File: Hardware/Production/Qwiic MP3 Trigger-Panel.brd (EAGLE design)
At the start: 115.6 x 115.8 mm, 636 parts, among them J1 MICRO-SD, J13 PTH, J14 QWIIC_RIGHT_ANGLE, J2 QWIIC_RIGHT_ANGLE, J20 MICRO-SD, J21 ISP, J22 Poke-Home, J23 3.5mm Audio, J25 QWIIC_RIGHT_ANGLE, J26 PTH, J27 QWIIC_RIGHT_ANGLE, J3 PTH, J32 MICRO-SD, J33 ISP, J34 Poke-Home, J35 3.5mm Audio, J37 QWIIC_RIGHT_ANGLE, J38 PTH, J39 QWIIC_RIGHT_ANGLE, J4 QWIIC_RIGHT_ANGLE, J44 MICRO-SD, J45 ISP, J46 Poke-Home, J47 3.5mm Audio, J49 QWIIC_RIGHT_ANGLE, J50 PTH, J51 QWIIC_RIGHT_ANGLE, J56 MICRO-SD, J57 ISP, J58 Poke-Home, J59 3.5mm Audio, J6 QWIIC_RIGHT_ANGLE, J61 QWIIC_RIGHT_ANGLE, J62 PTH, J63 QWIIC_RIGHT_ANGLE, J68 MICRO-SD, J69 ISP, J7 ISP, J70 Poke-Home, J71 3.5mm Audio, J8 3.5mm Audio, J9 Poke-Home, U1 TPA2005D1, U10 ATTINY84-ARDUINO, U11 AP2112-3.3V, U12 WT2003SH4, U13 TPA2005D1, U14 ATTINY84-ARDUINO, U15 AP2112-3.3V, U16 WT2003SH4, U17 TPA2005D1, U18 ATTINY84-ARDUINO, U19 AP2112-3.3V, U2 TPA2005D1, U20 WT2003SH4, U21 TPA2005D1, U22 ATTINY84-ARDUINO, U23 AP2112-3.3V, U24 WT2003SH4, U3 AP2112-3.3V, U4 ATTINY84-ARDUINO, U5 WT2003SH4, U6 ATTINY84-ARDUINO, U7 AP2112-3.3V, U8 WT2003SH4, U9 TPA2005D1

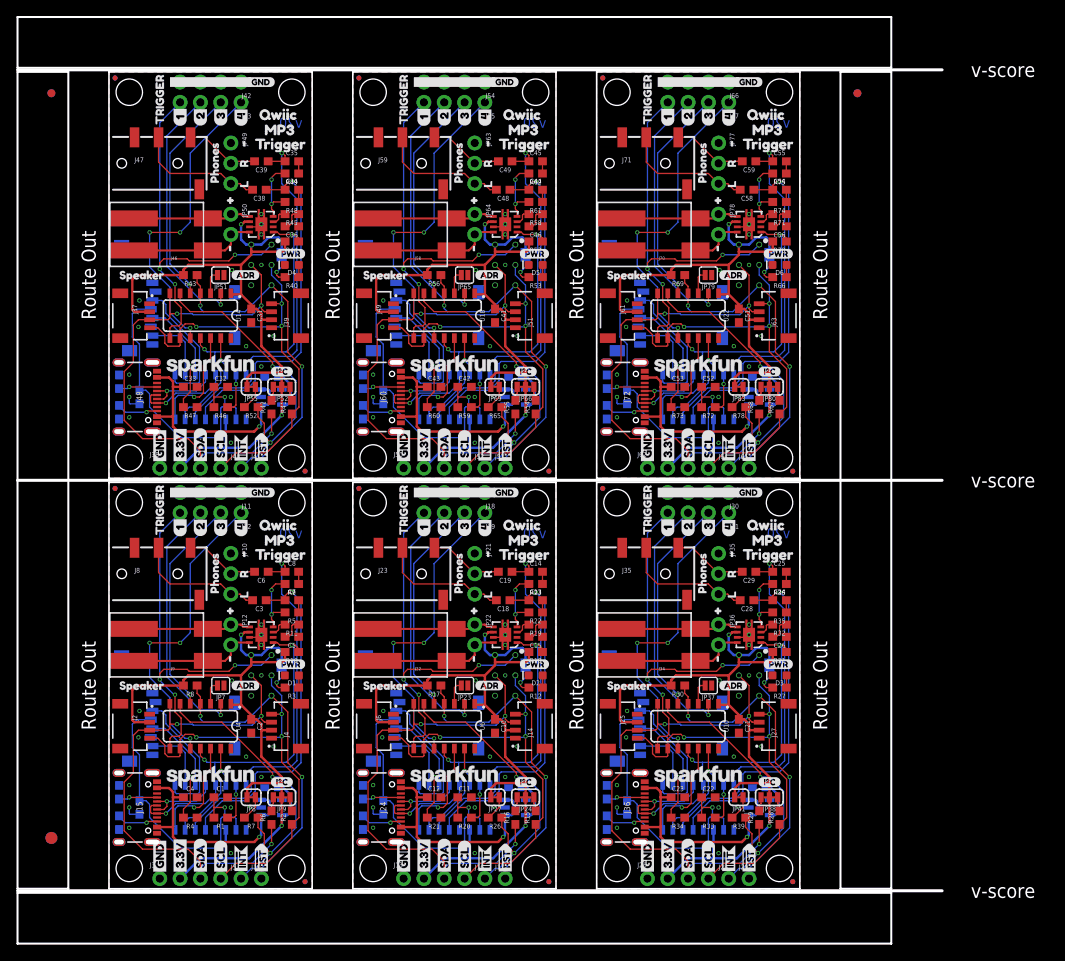
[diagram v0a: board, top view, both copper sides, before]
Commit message: v20 small test panel
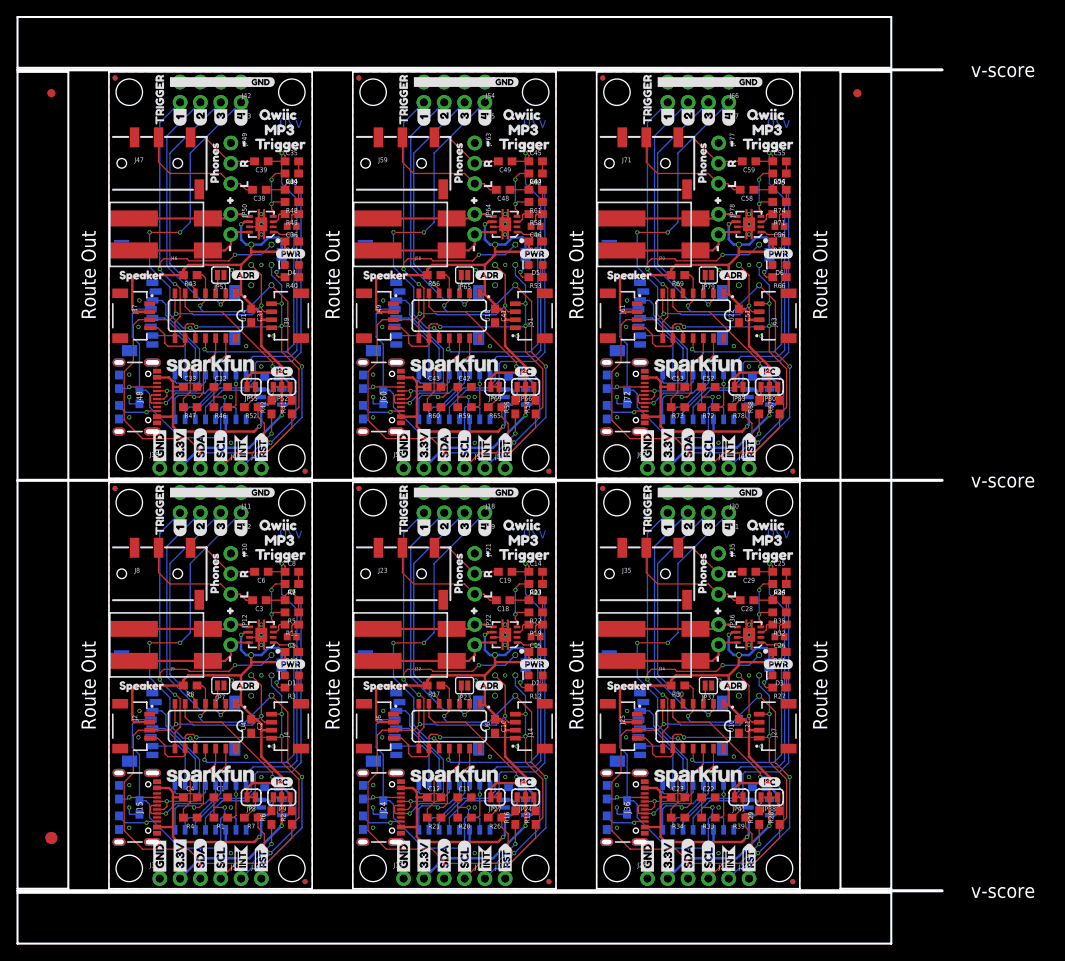
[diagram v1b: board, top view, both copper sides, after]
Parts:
- C13, C14, C24, C25, C34, C35, C44, C45, C54, C55, C7, C8: value 0.1uF -> 10nF
- C15, C26, C36, C46, C5, C56: value 1.0uF -> 22nF; device SparkFun-Capacitors:0603 -> SparkFun-Capacitors:0402
- R11, R19, R32, R45, R58, R71: value 100k -> 47k
- R17, R30, R43, R56, R69, R8: value 4.7k -> 10k
- R22, R23, R35, R36, R48, R49, R5, R61, R62, R74, R75, R9: value 10k -> 100k
- moved U10 0.64 mm to (73.0, 20.3)
- moved U18 0.64 mm to (42.5, 71.6)
- moved U22 0.64 mm to (73.0, 71.6)
- moved U6 0.64 mm to (42.5, 20.3)
- moved U14 0.63 mm to (12.1, 71.6)
- moved U4 0.63 mm to (12.1, 20.3)
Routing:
- net !RST2: track 41.3 -> 42.2 mm
- net !RST1: track 41.3 -> 42.2 mm
- net !RST5: track 41.3 -> 42.2 mm
- net !RST4: track 41.3 -> 42.2 mm
- net !RST3: track 41.3 -> 42.2 mm
- net !RST: track 41.3 -> 42.2 mm
- net TRIGGER22: track 48.7 -> 47.9 mm
- net TRIGGER10: track 48.7 -> 47.9 mm
- net TRIGGER1: track 48.7 -> 47.9 mm
- net TRIGGER6: track 48.7 -> 47.9 mm
- net TRIGGER18: track 48.7 -> 47.9 mm
- net TRIGGER14: track 48.7 -> 47.9 mm
- net 3.3V3: track 94.9 -> 94.2 mm
- net 3.3V2: track 94.9 -> 94.2 mm
- net 3.3V: track 94.9 -> 94.2 mm
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
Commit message: Proto with MY1690
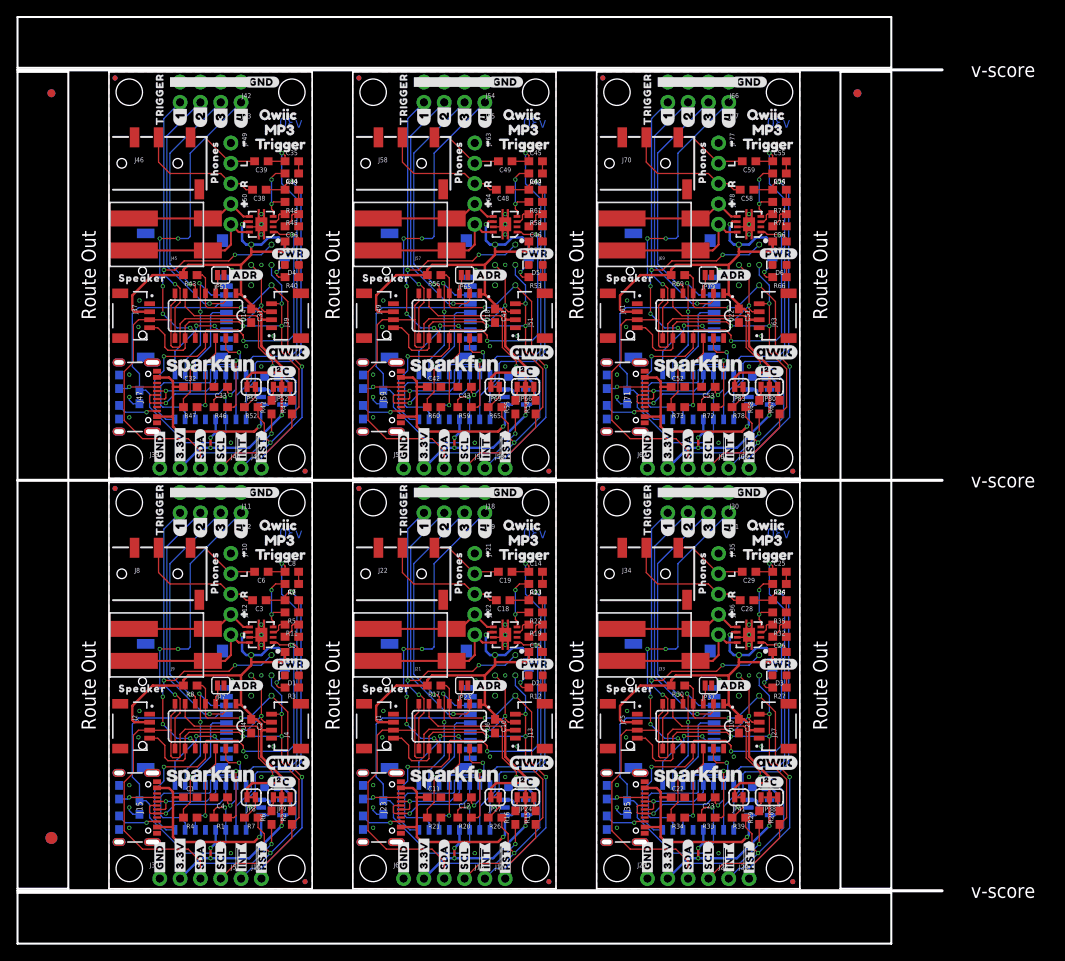
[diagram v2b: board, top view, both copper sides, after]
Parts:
- removed U$283: (no value), Labels:QWIIC-LOGO-MEDIUM
- removed U$284: (no value), buzzard_labels (2):TRIGGER4
- removed U$285: (no value), buzzard_labels (3):MP31
- removed U$286: (no value), buzzard_labels (3):QWIIC0
- removed U$287: (no value), buzzard_labels (3):TRIGGER2
- removed U$288: (no value), output:#PWR#0
- added LOGO19, LOGO23: SFE_LOGO_NAME_FLAME.1_INCH, SparkFun-Aesthetics:SFE_LOGO_NAME_FLAME_.1
- added LOGO20, LOGO24: QWIIC_LOGO_CONNECTOR, SparkFun-Aesthetics:QWIIC_5.5MM
- added LOGO21: OSHW-LOGOMINI, SparkFun-Aesthetics:OSHW-LOGO-MINI
- added LOGO22: SFE_LOGO_NAME.1_INCH, SparkFun-Aesthetics:SFE_LOGO_NAME_.1
- C1, C11, C22, C32, C42, C52: value 10uF -> 1.0uF
- C15, C26, C36, C46, C5, C56: device SparkFun-Capacitors:0402 -> SparkFun-Capacitors:0603
- J1: value MICRO-SD -> QWIIC_RIGHT_ANGLE; device SparkFun-Connectors:MICRO-SD-SOCKET -> SparkFun-Connectors:JST04_1MM_RA
- J13: value PTH -> QWIIC_RIGHT_ANGLE; device SparkX:1X04_NO_SILK -> SparkFun-Connectors:JST04_1MM_RA
- J14: value QWIIC_RIGHT_ANGLE -> MICRO-SD; device SparkFun-Connectors:JST04_1MM_RA -> SparkFun-Connectors:MICROSD-EXTERNALPIN
- J20, J32, J44, J56, J68: value MICRO-SD -> ISP; device SparkFun-Connectors:MICRO-SD-SOCKET -> SparkFun-Connectors:2X3_TEST_POINTS
- J21, J33, J45, J57, J69: value ISP -> Poke-Home; device SparkFun-Connectors:2X3_TEST_POINTS -> SparkFun-Connectors:1X02_POKEHOME
- J22, J34, J46, J58, J70: value Poke-Home -> 3.5mm Audio; device SparkFun-Connectors:1X02_POKEHOME -> SparkFun-Connectors:AUDIO_JACK_3.5MM_TRRS_SMD_RA
- J23, J35, J47, J59, J71: value 3.5mm Audio -> (none); device SparkFun-Connectors:AUDIO_JACK_3.5MM_TRRS_SMD_RA -> SparkFun-Connectors:USB-C-16P-2LAYER-PADS
- J24, J36, J48, J60, J72: value (none) -> MICRO-SD; device SparkFun-Connectors:USB-C-16P-2LAYER-PADS -> SparkFun-Connectors:MICROSD-EXTERNALPIN
- J6: value QWIIC_RIGHT_ANGLE -> PTH; device SparkFun-Connectors:JST04_1MM_RA -> SparkX:1X04_NO_SILK
- LOGO10: value OSHW-LOGOMINI -> SFE_LOGO_NAME.1_INCH; device SparkFun-Aesthetics:OSHW-LOGO-MINI -> SparkFun-Aesthetics:SFE_LOGO_NAME_.1
- LOGO11: value SFE_LOGO_NAME.1_INCH -> SFE_LOGO_NAME_FLAME.1_INCH; device SparkFun-Aesthetics:SFE_LOGO_NAME_.1 -> SparkFun-Aesthetics:SFE_LOGO_NAME_FLAME_.1
- LOGO12: value SFE_LOGO_NAME_FLAME.1_INCH -> QWIIC_LOGO_CONNECTOR; device SparkFun-Aesthetics:SFE_LOGO_NAME_FLAME_.1 -> SparkFun-Aesthetics:QWIIC_5.5MM
- LOGO16, LOGO4: value OSHW-LOGOMINI -> QWIIC_LOGO_CONNECTOR; device SparkFun-Aesthetics:OSHW-LOGO-MINI -> SparkFun-Aesthetics:QWIIC_5.5MM
- LOGO17, LOGO5: value SFE_LOGO_NAME.1_INCH -> OSHW-LOGOMINI; device SparkFun-Aesthetics:SFE_LOGO_NAME_.1 -> SparkFun-Aesthetics:OSHW-LOGO-MINI
- LOGO18, LOGO6: value SFE_LOGO_NAME_FLAME.1_INCH -> SFE_LOGO_NAME.1_INCH; device SparkFun-Aesthetics:SFE_LOGO_NAME_FLAME_.1 -> SparkFun-Aesthetics:SFE_LOGO_NAME_.1
- LOGO7: value OSHW-LOGOMINI -> SFE_LOGO_NAME_FLAME.1_INCH; device SparkFun-Aesthetics:OSHW-LOGO-MINI -> SparkFun-Aesthetics:SFE_LOGO_NAME_FLAME_.1
- LOGO8: value SFE_LOGO_NAME.1_INCH -> QWIIC_LOGO_CONNECTOR; device SparkFun-Aesthetics:SFE_LOGO_NAME_.1 -> SparkFun-Aesthetics:QWIIC_5.5MM
- LOGO9: value SFE_LOGO_NAME_FLAME.1_INCH -> OSHW-LOGOMINI; device SparkFun-Aesthetics:SFE_LOGO_NAME_FLAME_.1 -> SparkFun-Aesthetics:OSHW-LOGO-MINI
- U$10, U$38, U$69: device buzzard_labels (16):#6 -> output:#1#3
- U$100, U$148: device Labels-0_04:SDA8 -> output:#0
- U$101, U$194, U$242: device Labels-0_04:GND1 -> output:#0
- U$102, U$150: device Labels-0_04:3#3V2 -> output:#1
- U$103, U$196, U$244: device Labels-0_04:SDA8 -> output:#1
- U$104: device Labels-0_04:SCL9 -> output:QWIIC_MP30
- U$105: device Labels:I_SUPER2_C-()-03 -> output:TRIGGER1
- U$106: device Labels:INT#-[< -> output:#PWR#0
- U$107, U$154, U$155, U$202: device Labels:INT#-[< -> output:TRIGGER0
- U$108: device Labels:RST#-[> -> output:TRIGGER0
- U$109, U$156, U$157, U$204: device Labels:RST#-[> -> output:L1
- U$11: device Labels:INT#-[< -> output:#1
- U$110: device Labels:PWR-()-03 -> output:L1
- U$111, U$159: device Labels:ADR-()-03 -> output:R0
- U$112, U$64: device buzzard_labels (13):TRIGGER5 -> output:R0
- U$113, U$161: device buzzard_labels (14):21 -> output:#2
- U$114, U$66: device buzzard_labels (14):32 -> output:#2
- U$115, U$163: device buzzard_labels (14):43 -> output:#1#3
- U$116, U$68: device buzzard_labels (16):#5 -> output:#1#3
- U$117, U$165: device buzzard_labels (16):#6 -> output:#2#2
- U$118, U$70: device buzzard_labels (16):1_1 -> output:#2#2
- U$119, U$167: device buzzard_labels (16):GND0 -> output:#3#1
- U$12, U$28: device buzzard_labels (16):#5 -> output:#1
- U$120, U$72: device buzzard_labels (16):L12 -> output:#3#1
- U$121, U$169: device buzzard_labels (16):R11 -> output:#4#0
- U$122, U$74: device buzzard_labels (16):#6 -> output:#4#0
- U$123, U$171: device buzzard_labels (17):PHONES0 -> output:#GND#0
- U$124, U$76: device buzzard_labels (17):SPEAKER1 -> output:#GND#0
- U$125: device buzzard_labels (17):QWIIC_MP32 -> output:PHONES0
- U$126: device buzzard_labels (16):#6 -> output:#PWR#0
- U$127: device buzzard_labels (16):#5 -> output:#ADR#0
- U$128: device buzzard_labels (14):43 -> output:SPEAKER0
- U$129: device buzzard_labels (14):32 -> output:#I�C#0
- U$13: device buzzard_labels (16):#6 -> output:#1
- U$130, U$178: device buzzard_labels (16):#6 -> output:##INT##4
- U$131, U$83: device buzzard_labels (16):R11 -> output:##INT##4
- U$132, U$180: device buzzard_labels (16):L12 -> output:##RST##5
- U$133, U$85: device buzzard_labels (14):21 -> output:##RST##5
- U$134, U$182, U$44: device buzzard_labels (16):1_1 -> output:#3#3V#0
- U$135, U$87: device buzzard_labels (13):TRIGGER5 -> output:#3#3V#0
- U$136, U$184, U$46: device buzzard_labels (16):GND0 -> output:#GND#1
- U$137, U$89: device buzzard_labels (17):PHONES0 -> output:#GND#1
- U$138, U$186: device buzzard_labels (17):SPEAKER1 -> output:#SCL#3
- U$139, U$91: device Labels:QWIIC-LOGO-MEDIUM -> output:#SCL#3
- U$14: device buzzard_labels (17):SPEAKER1 -> output:#0
- U$140, U$188: device buzzard_labels (2):TRIGGER4 -> output:#SDA#2
- U$141, U$93: device buzzard_labels (3):MP31 -> output:#SDA#2
- U$142: device buzzard_labels (3):QWIIC0 -> buzzard_labels (3):MP31
- U$143: device buzzard_labels (3):TRIGGER2 -> buzzard_labels (3):QWIIC0
- U$144: device output:#PWR#0 -> buzzard_labels (3):TRIGGER2
- U$145: device Labels-0_04:3#3V2 -> output:PHONES0
- U$146: device Labels-0_04:GND1 -> output:SPEAKER0
- U$147, U$195, U$51: device Labels-0_04:SCL9 -> output:#0
- U$149, U$197: device Labels-0_04:GND1 -> output:#1
- U$15, U$267: device buzzard_labels (17):PHONES0 -> output:#PWR#0
- U$151: device Labels-0_04:SDA8 -> output:QWIIC_MP30
- U$152: device Labels-0_04:SCL9 -> output:TRIGGER1
- U$153: device Labels:I_SUPER2_C-()-03 -> output:#PWR#0
- U$158, U$206: device Labels:PWR-()-03 -> output:R0
- U$16: device Labels:RST#-[> -> output:QWIIC_MP30
- U$160, U$208: device buzzard_labels (13):TRIGGER5 -> output:#2
- U$162, U$210: device buzzard_labels (14):32 -> output:#1#3
- U$164, U$212: device buzzard_labels (16):#5 -> output:#2#2
- U$166, U$214: device buzzard_labels (16):1_1 -> output:#3#1
- U$168, U$216: device buzzard_labels (16):L12 -> output:#4#0
- U$17: device Labels:PWR-()-03 -> output:#ADR#0
- U$170, U$218: device buzzard_labels (16):#6 -> output:#GND#0
- U$172: device buzzard_labels (17):SPEAKER1 -> output:PHONES0
- U$173, U$24: device buzzard_labels (17):QWIIC_MP32 -> output:#PWR#0
- U$174: device buzzard_labels (16):#6 -> output:#ADR#0
- U$175: device buzzard_labels (16):#5 -> output:SPEAKER0
- U$176: device buzzard_labels (14):43 -> output:#I�C#0
- U$177, U$225, U$33: device buzzard_labels (14):32 -> output:##INT##4
- U$179, U$227: device buzzard_labels (16):R11 -> output:##RST##5
- U$18: device Labels:ADR-()-03 -> output:SPEAKER0
- U$181, U$229, U$42: device buzzard_labels (14):21 -> output:#3#3V#0
- U$183, U$231: device buzzard_labels (13):TRIGGER5 -> output:#GND#1
- U$185, U$233: device buzzard_labels (17):PHONES0 -> output:#SCL#3
- U$187, U$235: device Labels:QWIIC-LOGO-MEDIUM -> output:#SDA#2
- U$19: device buzzard_labels (16):1_1 -> output:#GND#0
- U$192: device output:#PWR#0 -> output:PHONES0
- U$193: device Labels-0_04:3#3V2 -> output:SPEAKER0
- U$198: device Labels-0_04:3#3V2 -> output:QWIIC_MP30
- U$199, U$52: device Labels-0_04:SDA8 -> output:TRIGGER1
- U$2: device output:#PWR#0 -> output:TRIGGER0
- U$20: device buzzard_labels (17):SPEAKER1 -> output:#I�C#0
- U$200: device Labels-0_04:SCL9 -> output:#PWR#0
- U$201, U$249: device Labels:I_SUPER2_C-()-03 -> output:TRIGGER0
- U$203, U$250, U$251: device Labels:INT#-[< -> output:L1
- U$205, U$252, U$253: device Labels:RST#-[> -> output:R0
- U$207, U$255: device Labels:ADR-()-03 -> output:#2
- U$209, U$257: device buzzard_labels (14):21 -> output:#1#3
- U$21, U$246: device Labels-0_04:3#3V2 -> output:TRIGGER1
- U$211, U$259: device buzzard_labels (14):43 -> output:#2#2
- U$213, U$261: device buzzard_labels (16):#6 -> output:#3#1
- U$215, U$263: device buzzard_labels (16):GND0 -> output:#4#0
- U$217, U$265: device buzzard_labels (16):R11 -> output:#GND#0
- U$219: device buzzard_labels (17):PHONES0 -> output:PHONES0
- U$22: device Labels-0_04:GND1 -> output:#PWR#0
- U$220: device buzzard_labels (17):SPEAKER1 -> output:#PWR#0
- U$221: device buzzard_labels (17):QWIIC_MP32 -> output:#ADR#0
- U$222: device buzzard_labels (16):#6 -> output:SPEAKER0
- U$223: device buzzard_labels (16):#5 -> output:#I�C#0
- U$224, U$272, U$34: device buzzard_labels (14):43 -> output:##INT##4
- U$226, U$274: device buzzard_labels (16):#6 -> output:##RST##5
- U$228, U$276: device buzzard_labels (16):L12 -> output:#3#3V#0
- U$230, U$278: device buzzard_labels (16):1_1 -> output:#GND#1
- U$232, U$280: device buzzard_labels (16):GND0 -> output:#SCL#3
- U$234, U$282: device buzzard_labels (17):SPEAKER1 -> output:#SDA#2
- U$236: device buzzard_labels (2):TRIGGER4 -> buzzard_labels (3):MP31
- U$237: device buzzard_labels (3):MP31 -> buzzard_labels (3):QWIIC0
- U$238: device buzzard_labels (3):QWIIC0 -> buzzard_labels (3):TRIGGER2
- U$239: device buzzard_labels (3):TRIGGER2 -> output:PHONES0
- U$240: device output:#PWR#0 -> output:SPEAKER0
- U$241: device Labels-0_04:3#3V2 -> output:#0
- U$243: device Labels-0_04:SCL9 -> output:#1
- U$245: device Labels-0_04:GND1 -> output:QWIIC_MP30
- U$247: device Labels-0_04:SDA8 -> output:#PWR#0
- U$248, U$26: device Labels-0_04:SCL9 -> output:TRIGGER0
- U$25: device buzzard_labels (16):#6 -> output:QWIIC_MP30
- U$254: device Labels:PWR-()-03 -> output:#2
- U$256: device buzzard_labels (13):TRIGGER5 -> output:#1#3
- U$258: device buzzard_labels (14):32 -> output:#2#2
- U$260: device buzzard_labels (16):#5 -> output:#3#1
- U$262: device buzzard_labels (16):1_1 -> output:#4#0
- U$264: device buzzard_labels (16):L12 -> output:#GND#0
- U$266, U$78: device buzzard_labels (16):#6 -> output:PHONES0
- U$268: device buzzard_labels (17):SPEAKER1 -> output:#ADR#0
- U$269: device buzzard_labels (17):QWIIC_MP32 -> output:SPEAKER0
- U$27: device Labels-0_04:SDA8 -> output:TRIGGER0
- U$270, U$82: device buzzard_labels (16):#6 -> output:#I�C#0
- U$271: device buzzard_labels (16):#5 -> output:##INT##4
- U$273, U$36: device buzzard_labels (14):32 -> output:##RST##5
- U$275: device buzzard_labels (16):R11 -> output:#3#3V#0
- U$277: device buzzard_labels (14):21 -> output:#GND#1
- U$279: device buzzard_labels (13):TRIGGER5 -> output:#SCL#3
- U$281: device buzzard_labels (17):PHONES0 -> output:#SDA#2
- U$29, U$45: device buzzard_labels (13):TRIGGER5 -> output:L1
- U$3: device Labels-0_04:GND1 -> buzzard_labels (3):MP31
- U$30: device Labels-0_04:3#3V2 -> output:L1
- U$31: device buzzard_labels (14):43 -> output:#GND#0
- U$32: device buzzard_labels (14):21 -> output:PHONES0
- U$35: device buzzard_labels (16):GND0 -> output:##RST##5
- U$37: device buzzard_labels (16):L12 -> output:R0
- U$39: device buzzard_labels (16):R11 -> output:R0
- U$4: device Labels-0_04:3#3V2 -> buzzard_labels (3):QWIIC0
- U$40: device buzzard_labels (17):PHONES0 -> output:SPEAKER0
- U$41: device buzzard_labels (16):L12 -> output:#2
- U$43: device buzzard_labels (16):R11 -> output:#2
- U$47: device Labels:QWIIC-LOGO-MEDIUM -> output:TRIGGER0
- U$48, U$98: device Labels-0_04:GND1 -> output:PHONES0
- U$49: device buzzard_labels (2):TRIGGER4 -> output:#2#2
- U$5: device Labels-0_04:SDA8 -> buzzard_labels (3):TRIGGER2
- U$53: device Labels-0_04:GND1 -> output:#2#2
- U$54: device Labels-0_04:3#3V2 -> output:#3#1
- U$55: device Labels-0_04:SDA8 -> output:#3#1
- U$56: device Labels-0_04:SCL9 -> output:#4#0
- U$57: device Labels:I_SUPER2_C-()-03 -> output:#4#0
- U$58: device Labels:INT#-[< -> output:#GND#1
- U$59: device Labels:INT#-[< -> output:#SCL#3
- U$6: device Labels-0_04:SCL9 -> output:PHONES0
- U$60: device Labels:RST#-[> -> output:#SCL#3
- U$61: device Labels:RST#-[> -> output:#SDA#2
- U$62: device Labels:PWR-()-03 -> output:#SDA#2
- U$63: device Labels:ADR-()-03 -> output:L1
- U$65: device buzzard_labels (14):21 -> output:R0
- U$67: device buzzard_labels (14):43 -> output:#2
- U$7: device Labels:RST#-[> -> output:SPEAKER0
- U$71: device buzzard_labels (16):GND0 -> output:#2#2
- U$73: device buzzard_labels (16):R11 -> output:#3#1
- U$75: device buzzard_labels (17):PHONES0 -> output:#4#0
- U$77: device buzzard_labels (17):QWIIC_MP32 -> output:#GND#0
- U$79: device buzzard_labels (16):#5 -> output:#PWR#0
- U$8: device Labels:I_SUPER2_C-()-03 -> output:#0
- U$80: device buzzard_labels (14):43 -> output:#ADR#0
- U$81: device buzzard_labels (14):32 -> output:SPEAKER0
- U$84: device buzzard_labels (16):L12 -> output:##INT##4
- U$86: device buzzard_labels (16):1_1 -> output:##RST##5
- U$88: device buzzard_labels (16):GND0 -> output:#3#3V#0
- U$9: device Labels:INT#-[< -> output:#0
- U$90: device buzzard_labels (17):SPEAKER1 -> output:#GND#1
- U$92: device buzzard_labels (2):TRIGGER4 -> output:#SCL#3
- U$94: device buzzard_labels (3):QWIIC0 -> output:#SDA#2
- U$95: device buzzard_labels (3):TRIGGER2 -> buzzard_labels (3):MP31
- U$96: device output:#PWR#0 -> buzzard_labels (3):QWIIC0
- U$97: device Labels-0_04:3#3V2 -> buzzard_labels (3):TRIGGER2
- U$99: device Labels-0_04:SCL9 -> output:SPEAKER0
- U12, U16, U20, U24, U8: value WT2003SH4 -> MY1690-16S; device SparkFun-IC-Special-Function:SO16 -> MY1690:SO16
- U2: value TPA2005D1 -> MY1690-16S; device SparkFun-IC-Amplifiers:QFN-8_PAD -> MY1690:SO16
- U5: value WT2003SH4 -> TPA2005D1; device SparkFun-IC-Special-Function:SO16 -> SparkFun-IC-Amplifiers:QFN-8_PAD
- moved LOGO12 104.9 mm to (83.3, 15.7), flipped to the top
- moved U$144 90.0 mm to (17.1, 93.1), flipped to the top, turned to 0 degrees
- moved U$143 81.7 mm to (17.7, 96.8)
- moved U$142 78.0 mm to (18.3, 94.9)
- moved LOGO10 67.0 mm to (73.7, 14.0), flipped to the top
- moved LOGO16 62.2 mm to (22.4, 67.1), flipped to the top
- moved LOGO11 61.7 mm to (67.8, 37.6), flipped to the bottom
- moved U$3 59.6 mm to (48.8, 43.6), flipped to the top, turned to 0 degrees
- moved U$4 58.8 mm to (48.1, 45.5), flipped to the top, turned to 0 degrees
- moved LOGO7 56.0 mm to (37.3, 37.6)
- moved U$22 54.8 mm to (52.5, 31.2), flipped to the bottom
- moved U$5 54.0 mm to (47.6, 41.8), flipped to the top, turned to 0 degrees
- moved U$27 52.3 mm to (36.8, 47.4)
- moved U$55 51.8 mm to (14.0, 45.2), flipped to the top
- moved U$56 51.8 mm to (16.5, 45.2), flipped to the top
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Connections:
- removed net N$13 (its old number): J24.B5, R24.2
- removed net N$21 (its old number): J36.B5, R37.2
- removed net N$22 (its old number): J36.A5, R38.2
- removed net N$29 (its old number): J48.B5, R50.2
- removed net N$30 (its old number): J48.A5, R51.2
- removed net N$37 (its old number): J60.B5, R63.2
- removed net N$38 (its old number): J60.A5, R64.2
- removed net N$46 (its old number): J72.A5, R77.2
- new net N$15: J23.A5, R25.2
- new net N$18: C12.1, U8.7
- new net N$23: J35.B5, R37.2
- new net N$24: J35.A5, R38.2
- new net N$27: C23.1, U12.7
- new net N$32: J47.B5, R50.2
- new net N$33: J47.A5, R51.2
- new net N$36: C33.1, U16.7
- new net N$41: J59.B5, R63.2
- new net N$42: J59.A5, R64.2
- new net N$50: J71.B5, R76.2
- new net N$51: J71.A5, R77.2
- new net N$54: C53.1, U24.7
- new net N$7: C4.1, U2.7
- net !RST1: now also J20.5; no longer J21.5
- net !RST2: now also J32.5; no longer J33.5
- net !RST3: now also J44.5; no longer J45.5
- net !RST4: now also J56.5; no longer J57.5
- net !RST5: now also J68.5; no longer J69.5
- net 3.3V: now also U2.12; no longer U5.11
- net 3.3V1: now also J1.2, J20.2, U5.6, U8.12; no longer J14.2, J21.2, U2.6, U8.11
- net 3.3V2: now also J32.2, U12.12; no longer J33.2, U12.11
- net 3.3V3: now also J44.2, U16.12; no longer J45.2, U16.11
- net 3.3V4: now also J56.2, U20.12; no longer J57.2, U20.11
- net 3.3V5: now also J68.2, U24.12; no longer J69.2, U24.11
- net 5V: now also C1.1; no longer C4.1
- net 5V1: now also C11.1, J23.VBUS1, J23.VBUS2; no longer C12.1, J24.VBUS1, J24.VBUS2
- net 5V2: now also C22.1, J35.VBUS1, J35.VBUS2; no longer C23.1, J36.VBUS1, J36.VBUS2
- net 5V3: now also C32.1, J47.VBUS1, J47.VBUS2; no longer C33.1, J48.VBUS1, J48.VBUS2
- net 5V4: now also C42.1, J59.VBUS1, J59.VBUS2; no longer C43.1, J60.VBUS1, J60.VBUS2
- net 5V5: now also C52.1, J71.VBUS1, J71.VBUS2; no longer C53.1, J72.VBUS1, J72.VBUS2
- net AC-L1: now also J22.RING1; no longer J23.RING1
- net AC-L2: now also J34.RING1; no longer J35.RING1
- net AC-L3: now also J46.RING1; no longer J47.RING1
- net AC-L4: now also J58.RING1; no longer J59.RING1
- net AC-L5: now also J70.RING1; no longer J71.RING1
- net AC-R1: now also J22.TIP; no longer J23.TIP
- net AC-R2: now also J34.TIP; no longer J35.TIP
- net AC-R3: now also J46.TIP; no longer J47.TIP
- net AC-R4: now also J58.TIP; no longer J59.TIP
- net AC-R5: now also J70.TIP; no longer J71.TIP
- net ADKEY: now also U2.4; no longer U5.7
- net ADKEY1: now also U8.4; no longer U8.7
- net ADKEY2: now also U12.4; no longer U12.7
- net ADKEY3: now also U16.4; no longer U16.7
- net ADKEY4: now also U20.4; no longer U20.7
- net ADKEY5: now also U24.4; no longer U24.7
- net D+: now also U2.6; no longer U5.5
- net D+1: now also J23.A6, J23.B6, U8.6; no longer J24.A6, J24.B6, U8.5
- net D+2: now also J35.A6, J35.B6, U12.6; no longer J36.A6, J36.B6, U12.5
- net D+3: now also J47.A6, J47.B6, U16.6; no longer J48.A6, J48.B6, U16.5
- net D+4: now also J59.A6, J59.B6, U20.6; no longer J60.A6, J60.B6, U20.5
- net D+5: now also J71.A6, J71.B6, U24.6; no longer J72.A6, J72.B6, U24.5
- net D-: now also U2.5; no longer U5.4
- net D-1: now also J23.A7, J23.B7, U8.5; no longer J24.A7, J24.B7, U8.4
- net D-2: now also J35.A7, J35.B7, U12.5; no longer J36.A7, J36.B7, U12.4
- net D-3: now also J47.A7, J47.B7, U16.5; no longer J48.A7, J48.B7, U16.4
- net D-4: now also J59.A7, J59.B7, U20.5; no longer J60.A7, J60.B7, U20.4
- net D-5: now also J71.A7, J71.B7, U24.5; no longer J72.A7, J72.B7, U24.4
- net GND: now also J14.10, J14.11, J14.12, J14.13, J14.6, U2.13, U2.8; no longer J1.CD1, J1.GND, U5.12, U5.8
- net GND1: now also J1.1, J20.6, J22.EARTH, J22.RING2, J23.GND, J23.GND2, J23.SHLD1, J23.SHLD2, J23.SHLD3, J23.SHLD4, J24.10, J24.11, J24.12, J24.13, J24.6, U5.10, U5.11, U5.12, U5.13, U5.7, U5.9, U8.13; no longer J14.1, J20.CD1, J20.GND, J21.6, J23.EARTH, J23.RING2, J24.GND, J24.GND2, J24.SHLD1, J24.SHLD2, J24.SHLD3, J24.SHLD4, U2.10, U2.11, U2.12, U2.13, U2.7, U2.9, U8.12
- net GND2: now also J32.6, J34.EARTH, J34.RING2, J35.GND, J35.GND2, J35.SHLD1, J35.SHLD2, J35.SHLD3, J35.SHLD4, J36.10, J36.11, J36.12, J36.13, J36.6, U12.13; no longer J32.CD1, J32.GND, J33.6, J35.EARTH, J35.RING2, J36.GND, J36.GND2, J36.SHLD1, J36.SHLD2, J36.SHLD3, J36.SHLD4, U12.12
- net GND3: now also J44.6, J46.EARTH, J46.RING2, J47.GND, J47.GND2, J47.SHLD1, J47.SHLD2, J47.SHLD3, J47.SHLD4, J48.10, J48.11, J48.12, J48.13, J48.6, U16.13; no longer J44.CD1, J44.GND, J45.6, J47.EARTH, J47.RING2, J48.GND, J48.GND2, J48.SHLD1, J48.SHLD2, J48.SHLD3, J48.SHLD4, U16.12
- net GND4: now also J56.6, J58.EARTH, J58.RING2, J59.GND, J59.GND2, J59.SHLD1, J59.SHLD2, J59.SHLD3, J59.SHLD4, J60.10, J60.11, J60.12, J60.13, J60.6, U20.13; no longer J56.CD1, J56.GND, J57.6, J59.EARTH, J59.RING2, J60.GND, J60.GND2, J60.SHLD1, J60.SHLD2, J60.SHLD3, J60.SHLD4, U20.12
- net GND5: now also J68.6, J70.EARTH, J70.RING2, J71.GND, J71.GND2, J71.SHLD1, J71.SHLD2, J71.SHLD3, J71.SHLD4, J72.10, J72.11, J72.12, J72.13, J72.6, U24.13; no longer J68.CD1, J68.GND, J69.6, J71.EARTH, J71.RING2, J72.GND, J72.GND2, J72.SHLD1, J72.SHLD2, J72.SHLD3, J72.SHLD4, U24.12
- net IN+AMP1: now also U5.3; no longer U2.3
- net IN-AMP1: now also U5.4; no longer U2.4
- net MP3-RXI: now also U2.15; no longer U5.6
- net MP3-RXI1: now also U8.15; no longer U8.6
- net MP3-RXI2: now also U12.15; no longer U12.6
- net MP3-RXI3: now also U16.15; no longer U16.6
- net MP3-RXI4: now also U20.15; no longer U20.6
- net MP3-RXI5: now also U24.15; no longer U24.6
- net MP3-TXO: now also U2.14; no longer U5.16
- net MP3-TXO1: now also U8.14; no longer U8.16
- net MP3-TXO2: now also U12.14; no longer U12.16
- net MP3-TXO3: now also U16.14; no longer U16.16
- net MP3-TXO4: now also U20.14; no longer U20.16
- net MP3-TXO5: now also U24.14; no longer U24.16
- net N$14: now also J23.B5, R24.2; no longer J24.A5, R25.2
- net N$45: now also C43.1, U20.7; no longer J72.B5, R76.2
- net OUT+1: now also J21.P1, J21.P3, U5.5; no longer J22.P1, J22.P3, U2.5
- net OUT+2: now also J33.P1, J33.P3; no longer J34.P1, J34.P3
- net OUT+3: now also J45.P1, J45.P3; no longer J46.P1, J46.P3
- net OUT+4: now also J57.P1, J57.P3; no longer J58.P1, J58.P3
- net OUT+5: now also J69.P1, J69.P3; no longer J70.P1, J70.P3
- net OUT-1: now also J21.P2, J21.P4, U5.8; no longer J22.P2, J22.P4, U2.8
- net OUT-2: now also J33.P2, J33.P4; no longer J34.P2, J34.P4
- net OUT-3: now also J45.P2, J45.P4; no longer J46.P2, J46.P4
- net OUT-4: now also J57.P2, J57.P4; no longer J58.P2, J58.P4
- net OUT-5: now also J69.P2, J69.P4; no longer J70.P2, J70.P4
- net PLAYING: now also U2.16; no longer U5.15
- net PLAYING1: now also U5.1, U8.16; no longer U2.1, U8.15
- net PLAYING2: now also U12.16; no longer U12.15
- net PLAYING3: now also U16.16; no longer U16.15
- net PLAYING4: now also U20.16; no longer U20.15
- net PLAYING5: now also U24.16; no longer U24.15
- net SCL1: now also J1.4, J20.3; no longer J14.4, J21.3
- net SCL2: now also J32.3; no longer J33.3
- net SCL3: now also J44.3; no longer J45.3
- net SCL4: now also J56.3; no longer J57.3
- net SCL5: now also J68.3; no longer J69.3
- net SDA1: now also J1.3, J20.4; no longer J14.3, J21.4
- net SDA2: now also J32.4; no longer J33.4
- net SDA3: now also J44.4; no longer J45.4
- net SDA4: now also J56.4; no longer J57.4
- net SDA5: now also J68.4; no longer J69.4
- net SD_CLK: now also J14.5, U2.3; no longer J1.SCLK, U5.3
- net SD_CLK1: now also J24.5; no longer J20.SCLK
- net SD_CLK2: now also J36.5; no longer J32.SCLK
- net SD_CLK3: now also J48.5; no longer J44.SCLK
- net SD_CLK4: now also J60.5; no longer J56.SCLK
- net SD_CLK5: now also J72.5; no longer J68.SCLK
- net SD_CMD: now also J14.3, U2.2; no longer J1.DI, U5.1
- net SD_CMD1: now also J24.3, U8.2; no longer J20.DI, U8.1
- net SD_CMD2: now also J36.3, U12.2; no longer J32.DI, U12.1
- net SD_CMD3: now also J48.3, U16.2; no longer J44.DI, U16.1
- net SD_CMD4: now also J60.3, U20.2; no longer J56.DI, U20.1
- net SD_CMD5: now also J72.3, U24.2; no longer J68.DI, U24.1
- net SD_DAT: now also J14.7, U2.1; no longer J1.DO, U5.2
- net SD_DAT1: now also J24.7, U8.1; no longer J20.DO, U8.2
- net SD_DAT2: now also J36.7, U12.1; no longer J32.DO, U12.2
- net SD_DAT3: now also J48.7, U16.1; no longer J44.DO, U16.2
- net SD_DAT4: now also J60.7, U20.1; no longer J56.DO, U20.2
- net SD_DAT5: now also J72.7, U24.1; no longer J68.DO, U24.2
- net TRIGGER10: now also J32.1; no longer J33.1
- net TRIGGER14: now also J44.1; no longer J45.1
- net TRIGGER18: now also J56.1; no longer J57.1
- net TRIGGER22: now also J68.1; no longer J69.1
- net TRIGGER6: now also J20.1; no longer J21.1
- net VCCIO: now also J14.4, U2.11; no longer C1.1, J1.VCC, U5.10
- net VCCIO1: now also J24.4, U8.11; no longer C11.1, J20.VCC, U8.10
- net VCCIO2: now also J36.4, U12.11; no longer C22.1, J32.VCC, U12.10
- net VCCIO3: now also J48.4, U16.11; no longer C32.1, J44.VCC, U16.10
- net VCCIO4: now also J60.4, U20.11; no longer C42.1, J56.VCC, U20.10
- net VCCIO5: now also J72.4, U24.11; no longer C52.1, J68.VCC, U24.10
- net VOUTL: now also U2.9; no longer U5.13
- net VOUTL1: now also U8.9; no longer U8.13
- net VOUTL2: now also U12.9; no longer U12.13
- net VOUTL3: now also U16.9; no longer U16.13
- net VOUTL4: now also U20.9; no longer U20.13
- net VOUTL5: now also U24.9; no longer U24.13
- net VOUTR: now also U2.10; no longer U5.14
- net VOUTR1: now also U8.10; no longer U8.14
- net VOUTR2: now also U12.10; no longer U12.14
- net VOUTR3: now also U16.10; no longer U16.14
- net VOUTR4: now also U20.10; no longer U20.14
- net VOUTR5: now also U24.10; no longer U24.14
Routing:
- net MP3-RXI5: track 5.09 -> 23.4 mm
- net MP3-RXI2: track 5.09 -> 23.4 mm
- net MP3-RXI4: track 5.09 -> 23.4 mm
- net MP3-RXI3: track 5.09 -> 23.4 mm
- net MP3-RXI1: track 5.09 -> 23.4 mm
- net MP3-RXI: track 5.09 -> 23.4 mm
- net SDA1: track 66.7 -> 74.0 mm
- net SDA5: track 66.7 -> 74.0 mm
- net SDA4: track 66.7 -> 74.0 mm
- net SDA2: track 66.7 -> 74.0 mm
- net SDA3: track 66.7 -> 74.0 mm
- net SDA: track 66.7 -> 74.0 mm
- net ADKEY3: track 4.98 -> 11.9 mm
- net ADKEY4: track 4.98 -> 11.9 mm
- net ADKEY5: track 4.98 -> 11.9 mm
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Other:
- board text added: "v30"
- board text removed: "v20"
